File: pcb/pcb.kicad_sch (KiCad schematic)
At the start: 8 parts, among them J1 Conn_01x04_Pin, J2 Conn_01x06_Pin, U1 XIAO-ESP32-C5-DIP, U17 AP2112K-3.3

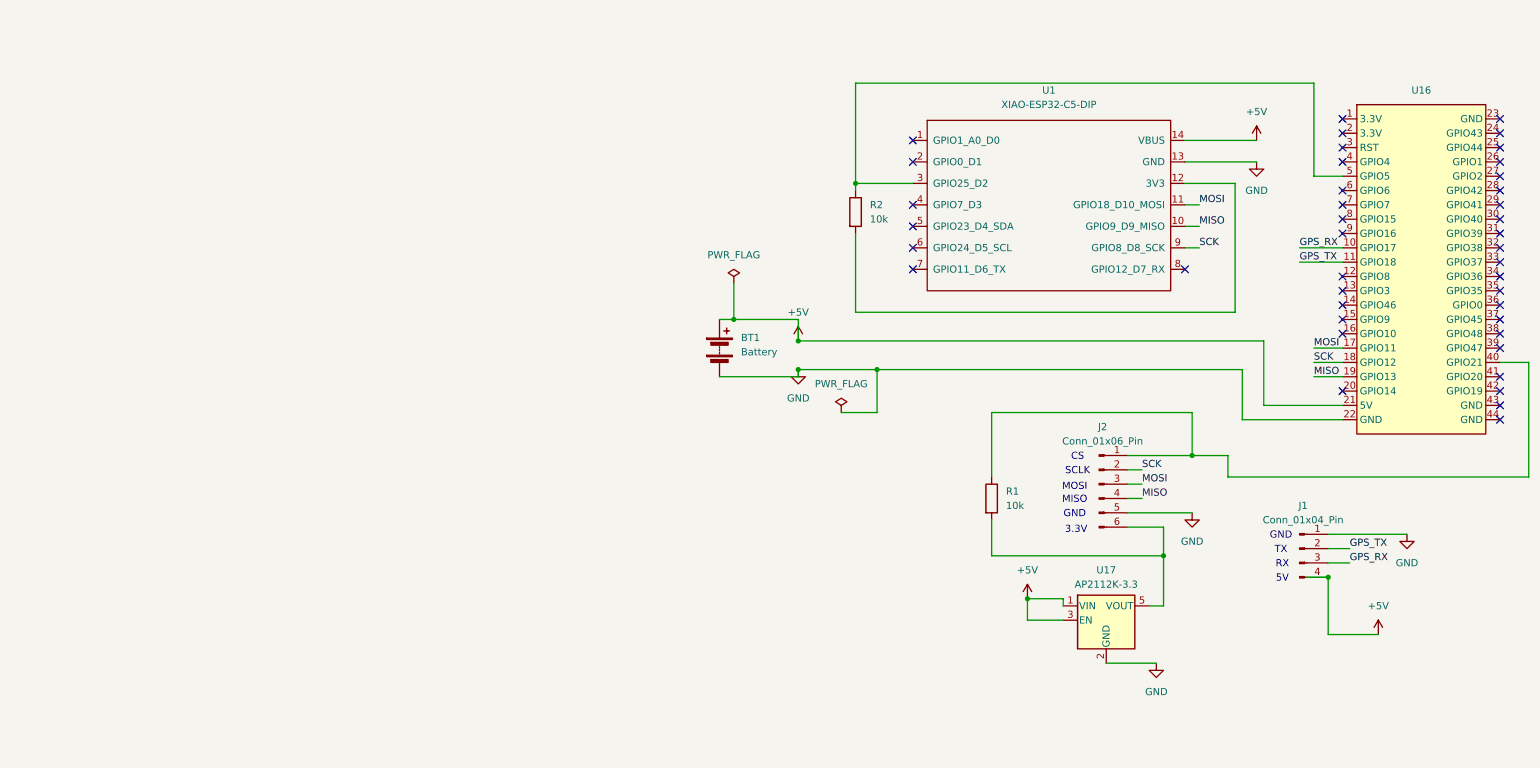
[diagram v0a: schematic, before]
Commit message: tidy schematic
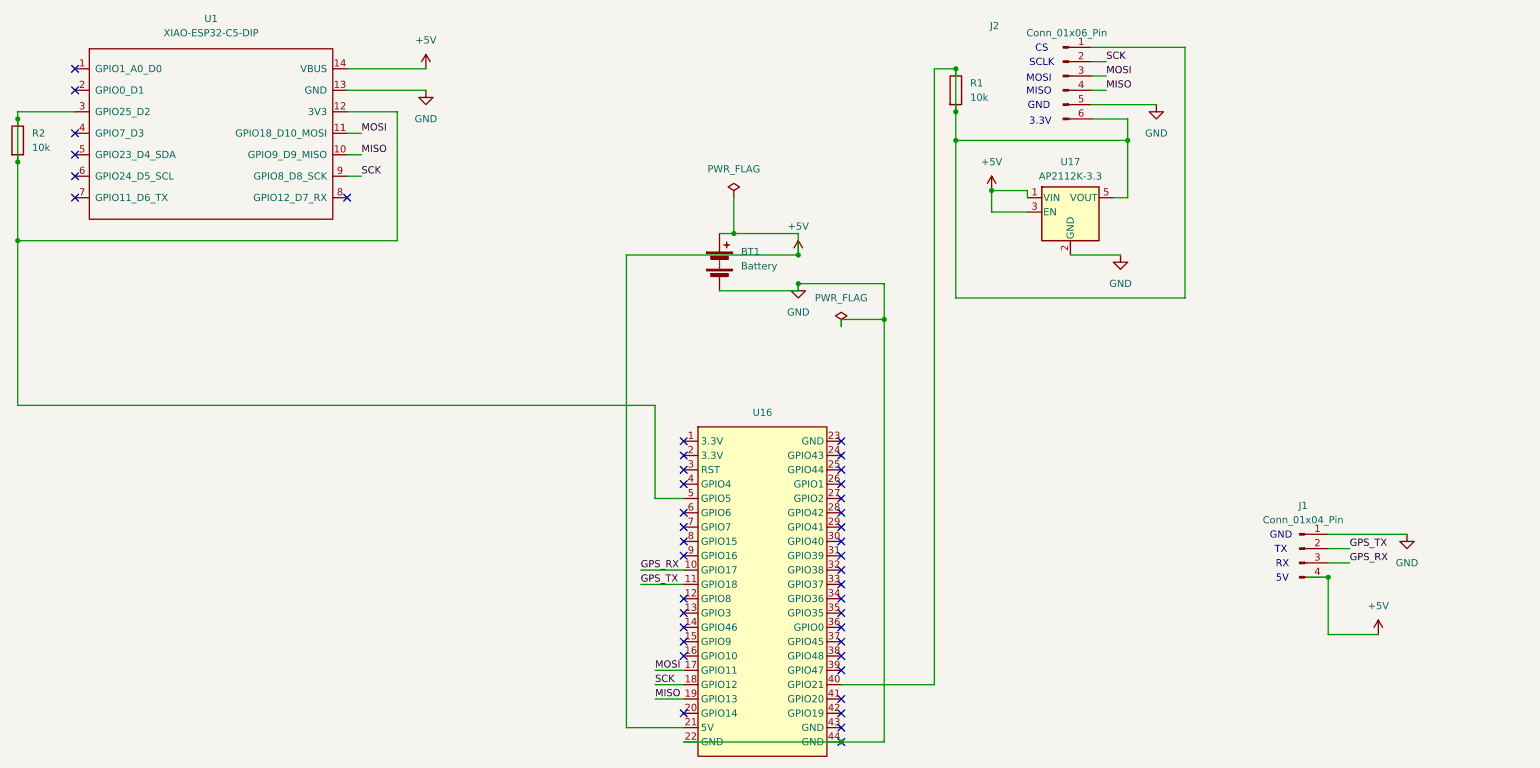
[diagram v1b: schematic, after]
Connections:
- net GND: now also U16.44 (GND)
- net at J2.1 (Pin_1), R1.1, U16.40 (GPIO21): now also J2.6 (Pin_6), R1.2, U17.5 (VOUT)
- net at R2.1, U1.3 (GPIO25_D2), U16.5 (GPIO5): now also R2.2, U1.12 (3V3)
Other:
- moved on the sheet: BT1, J2, R1, R2, U1, U16, U17
